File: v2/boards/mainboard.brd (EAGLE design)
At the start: 119.6 x 119.8 mm, 197 parts, among them IC1 LM2596S-ADJ, IC10 DRV8835, IC11 TSOP324, IC12 ESP-WROOM-32, IC13 PAM8403, IC15 MC1525, IC16 INA282, IC17 INA282, IC18 INA282, IC19 INA282, IC2 LM2596S-5.0, IC20 MCP3008, IC3 LD1117A, IC4 LM393, IC7 PCA9634, IC8 PCA9554, IC9 PCA9634, J1 Bat_In, J10 SPI_0, J11 SPI_2, J12 SPI_2, J13 I2C_0, J14 I2C_1, J15 I2C_3, J16 BNO055, J17 Uart_2, J18 Uart_5, J19 Uart_6 (LP), J2 Erw_Pwr, J20 BPS, J21 Servo_2, J22 Servo_3, J23 Erw_Servo, J24 Erw_PWM, J25 ESP32_Uart, J26 SPEAKER_L, J27 SPEAKER_R, J28 AUDIO_TEENSY, J29 SWD, J3 I2C0_5V, J30 SWD_KL02, J31 Erw_ENA, J32 Erw_GPIO, J33 Erw_analog, J34 RC5, J35 ESP32_PROG, J36 SPI1, J4 I2C3_5V, J5 Servo_1, J6 H-Bridge Mode, J7 ESP32_GPIO, J8 SPI_0, J9 SPI_0, SW1 TL32PO, U1 IRLU024N, U5 BS108, U6 BS108, U7 BS108, U8 BS108, U9 BS108, X1 max. 18V

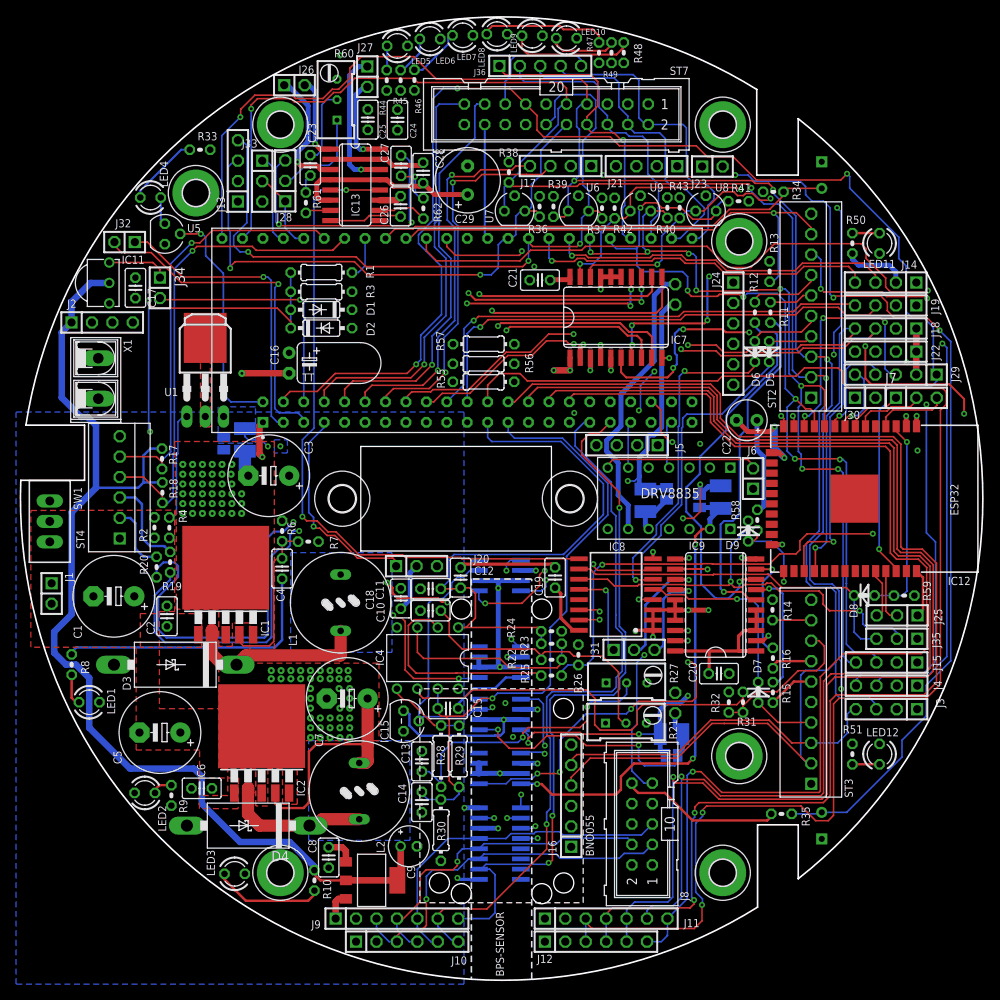
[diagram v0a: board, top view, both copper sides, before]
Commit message: schematics and board files for ct-Bot v2 prototype
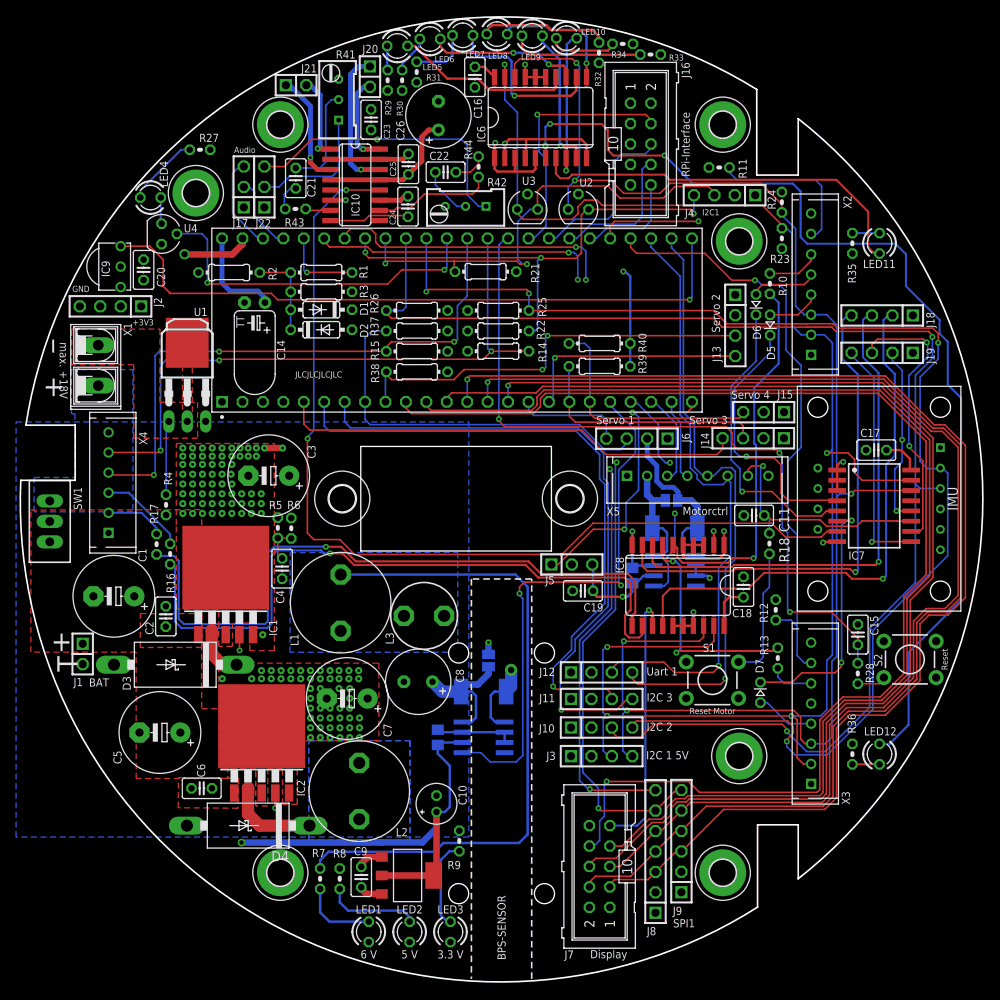
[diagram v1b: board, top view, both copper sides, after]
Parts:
- removed C27: 470nF, rcl:C025-025X050
- removed C28: 1uF, rcl:C025-025X050
- removed C29: 470uF, rcl:E3,5-8
- removed D8, D9: BAT42, ct-bot:0207/2V
- removed IC11: TSOP324, ct-bot:TSOP324
- removed IC12: ESP-WROOM-32, ct-bot:ESP-WROOM-32
- removed IC13: PAM8403, ct-bot:SOP-16
- removed IC15: MC1525, ct-bot:TO92
- removed IC16, IC17, IC18, IC19: INA282, ct-bot:SO08
- removed IC20: MCP3008, ct-bot:SO16
- removed J23: Erw_Servo, ct-bot:1X02
- removed J24: Erw_PWM, ct-bot:1X06
- removed J25: ESP32_Uart, ct-bot:1X03
- removed J26: SPEAKER_L, ct-bot:1X02
- removed J27: SPEAKER_R, ct-bot:1X02
- removed J28: AUDIO_TEENSY, ct-bot:1X03
- removed J29: SWD, ct-bot:1X05
- removed J30: SWD_KL02, ct-bot:1X02
- removed J31: Erw_ENA, ct-bot:1X03
- removed J32: Erw_GPIO, ct-bot:1X02
- removed J33: Erw_analog, ct-bot:1X03
- removed J34: RC5, ct-bot:1X02
- removed J35: ESP32_PROG, ct-bot:1X03
- removed J36: SPI1, ct-bot:1X05
- removed LDR1, LDR2: (no value), ct-bot:SNR2-3.0
- removed R45: 3k9, rcl:0204V
- removed R46: 220, rcl:0204V
- removed R47: 590, rcl:0204V
- removed R48: 115, rcl:0204V
- removed R49: 1k8, rcl:0204V
- removed R50, R51: 4k7, rcl:0204V
- removed R52, R53, R54: 20m, rcl:R1210
- removed R55, R56, R57: 4k7, rcl:0204/7
- removed R58, R59, R61, R62: 10k, rcl:0204V
- removed R60: 5k, ct-bot:RTRIM64W
- removed SJ3, SJ4: (no value), jumper:SJ
- removed ST1: CTBOT_MCU_BRD, ct-bot:DIP66
- removed ST2: Sensoren L, ct-bot:TS_PS25_10
- removed ST3: Sensoren R, ct-bot:TS_PS25_10
- removed ST4: Liniensensoren, ct-bot:TS_PS25_6
- removed ST5: Motor R, ct-bot:1X02/90
- removed ST6: Motor L, ct-bot:1X02/90
- removed ST7: RPI_Interface, con-harting-ml:ML20
- removed U5, U6, U7, U8, U9: BS108, ct-bot:SOT54E
- added IC5: (no value), ct-bot:SO08
- added IC6: PCA9634, ct-bot:SO20W
- added L3: 3u3, ct-bot:FASTRON_07HCP_INDUCTOR
- added MCU: CTBOT_MCU_BRD_V2, ct-bot:DIP48
- added S1, S2: Reset, SparkFun-Switches:TACTILE_SWITCH_PTH_6.0MM
- added U$10: IMU, ct-bot:NXP_9DOF
- added U2, U3, U4: BS108, ct-bot:SOT54E
- added X2: Sensoren L, ct-bot:B8B-XH
- added X3: Sensoren R, ct-bot:B8B-XH
- added X4: Liniensensoren, ct-bot:B6B-XH
- added X5: Motorctrl, ct-bot:B8B-XH
- C10: value 100nF -> 10uF; device rcl:C025-025X050 -> rcl:E2-5
- C11: value 2.2nF -> 1nF
- C12: value 6.8nF -> 100nF; device rcl:C025-025X050 -> rcl:C0805
- C13: device rcl:C025-025X050 -> rcl:C0805
- C14: value 2.2nF -> 10uF; device rcl:C025-025X050 -> rcl:TT2D5L
- C15: value 6.8nF -> 1nF
- C16: value 10uF -> 100nF; device rcl:TT2D5L -> rcl:C025-025X050
- C21: value 100nF -> 470nF
- C22: value 10uF -> 470nF; device rcl:E2,5-5 -> rcl:C025-025X050
- C23: value 470nF -> 1uF
- C24: value 1uF -> 100nF
- C26: value 100nF -> 470uF; device rcl:C025-025X050 -> rcl:E3,5-8
- C3: value 220u -> 220uF
- C7: value 680uF -> 220uF
- C8: value 100nF -> 180uF; device rcl:C025-025X050 -> rcl:E3,5-8
- C9: value 10uF -> 100nF; device rcl:E2-5 -> rcl:C025-025X050
- IC10: value DRV8835 -> PAM8403; device ct-bot:DRV8835 -> ct-bot:SOP-16
- IC4: value LM393 -> (none); device linear:DIL08 -> ct-bot:SO08
- IC7: value PCA9634 -> PCA9554; device ct-bot:SO20W -> ct-bot:SO16W
- IC8: value PCA9554 -> PCA9634; device ct-bot:SO16W -> ct-bot:SO20W
- IC9: value PCA9634 -> TSOP324; device ct-bot:SO20W -> ct-bot:TSOP324
- J10: value SPI_0 -> I2C_2; device ct-bot:1X06 -> ct-bot:1X04
- J11: value SPI_2 -> I2C_3; device ct-bot:1X07 -> ct-bot:1X04
- J12: value SPI_2 -> Uart_1; device ct-bot:1X06 -> ct-bot:1X04
- J13: value I2C_0 -> Servo_2
- J14: value I2C_1 -> Servo_3
- J15: value I2C_3 -> Servo_4; device ct-bot:1X04 -> ct-bot:1X03
- J16: value BNO055 -> RPi_Interface; device ct-bot:1X06 -> con-harting-ml:ML10
- J17: value Uart_2 -> Audio; device ct-bot:1X04 -> ct-bot:1X03
- J18: value Uart_5 -> Erw_DRV
- J19: value Uart_6 (LP) -> Erw_ENA
- J20: value BPS -> SPEAKER_R; device ct-bot:1X03 -> ct-bot:1X02
- J21: value Servo_2 -> SPEAKER_L; device ct-bot:1X04 -> ct-bot:1X02
- J22: value Servo_3 -> AUDIO_IN; device ct-bot:1X04 -> ct-bot:1X03
- J3: value I2C0_5V -> I2C1_5V
- J4: value I2C3_5V -> I2C_1
- J5: value Servo_1 -> BPS; device ct-bot:1X04 -> ct-bot:1X03
- J6: value H-Bridge Mode -> Servo_1; device ct-bot:1X02 -> ct-bot:1X04
- J7: value ESP32_GPIO -> SPI_1; device ct-bot:1X03 -> con-harting-ml:ML10
- J8: value SPI_0 -> SPI_1; device con-harting-ml:ML10 -> ct-bot:1X07
- J9: value SPI_0 -> SPI_1; device ct-bot:1X07 -> ct-bot:1X06
- R10: value 120 -> 180
- R11, R12: value 180 -> 47k
- R13, R17: value 47k -> 180
- R14, R2, R37: device rcl:0204V -> rcl:0204/7
- R15: value 180 -> 47k; device rcl:0204V -> rcl:0204/7
- R18: value 47k -> 330
- R19: value 180 -> 30m; device rcl:0204V -> rcl:R2512
- R20: value 180 -> 100m; device rcl:0204V -> rcl:R2512
- R21: value 5k -> 4k7; device ct-bot:RTRIM64W -> rcl:0204/7
- R22, R38, R39: value 10k -> 4k7; device rcl:0204V -> rcl:0204/7
- R23: value 1M -> 10k
- R25: value 10k -> 1k1; device rcl:0204V -> rcl:0204/7
- R26: value 15k -> 1k1; device rcl:0204V -> rcl:0204/7
- R27: value 5k -> 1k8; device ct-bot:RTRIM64W -> rcl:0204V
- R28: value 10k -> 330; device rcl:0204/7 -> rcl:0204V
- R29: value 1M -> 27k; device rcl:0204/7 -> rcl:0204V
- R30: device rcl:0204/7 -> rcl:0204V
- R31: value 10k -> 15k
- R32: value 15k -> 2k2
- R33: value 100 -> 2k2
- R34: value 470k -> 1k8
- R35: value 470k -> 10k
- R36, R44: value 4k7 -> 10k
- R40: value 1k1 -> 4k7; device rcl:0204V -> rcl:0204/7
- R41: value 1k1 -> 5k; device rcl:0204V -> ct-bot:RTRIM64W
- R42: value 1k8 -> 5k; device rcl:0204V -> ct-bot:RTRIM64W
- R43: value 1k8 -> 10k
- R5: value 20m -> 3k9 0.1%; device rcl:R1210 -> rcl:0204V
- R6: value 3k9 0.1% -> 1k 0.1%
- R7: value 1k 0.1% -> 27k
- R8: value 390 -> 22k
- R9: value 330 -> 15k
- moved C17 94.3 mm to (46.6, 6.05), turned to 180 degrees
- moved R30 93.3 mm to (-12.4, 52.0), turned to 90 degrees
- moved R10 93.3 mm to (33.4, 26.7), turned to 270 degrees
- moved R31 88.2 mm to (-10.6, 53.0), turned to 90 degrees
- moved C20 87.4 mm to (-44.5, 28.4), turned to 270 degrees
- moved IC9 85.1 mm to (-47.3, 28.9), turned to 270 degrees
- moved R27 84.6 mm to (-37.5, 43.4), turned to 0 degrees
- moved R29 84.5 mm to (-14.2, 52.0), turned to 90 degrees
- moved R32 82.3 mm to (12.1, 55.4)
- moved J16 81.5 mm to (17.3, 44.1), turned to 270 degrees
- moved J22 79.9 mm to (-29.5, 38.8), turned to 90 degrees
- moved R36 78.4 mm to (43.6, -31.8), turned to 270 degrees
- moved R16 76.0 mm to (-41.2, -6.87)
- moved R18 75.7 mm to (33.3, -5.58)
- moved R35 71.5 mm to (43.6, 31.8), turned to 90 degrees
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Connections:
- net V5_L1 renamed V5_L2
- removed net A22_DAC1: J33.1, ST1.48
- removed net AUDIO_OUT: J28.1, J33.2, ST1.49
- removed net BAT_CUR: IC17.5, IC20.1
- removed net BNO055_RESET: IC8.7, J16.6
- removed net DRV_RADLED_L: IC9.6, R11.2
- removed net DRV_RADLED_R: IC9.7, R15.1
- removed net EN: D8.1, IC12.3, R59.1
- removed net ENC_L: R25.2, R26.1, ST2.8
- removed net ENC_R: R31.2, R32.1, ST3.8
- removed net ESP32_PROG: D9.2, IC8.11, J35.2
- removed net ESP32_RESET: D8.2, IC8.10, J35.3
- removed net GND_BAT: IC17.1, R5.2, SJ1.2, U1.3
- removed net GPIO_24: J32.1, ST1.2
- removed net GPIO_46: J32.2, ST1.3
- removed net IO0: D9.1, IC12.25, R58.2
- removed net IO10: IC12.18
- removed net IO11: IC12.19
- removed net IO13: IC12.16
- removed net IO15: IC12.23
- removed net IO18: IC12.30
- removed net IO19: IC12.31
- removed net IO21: IC12.33
- removed net IO34: IC12.6, J7.2
- removed net IO35: IC12.7, J7.1
- removed net IO36: IC12.4, J7.3
- removed net IO39: IC12.5
- removed net IO4: IC12.26
- removed net IO5: IC12.29
- removed net IO6: IC12.20
- removed net IO7: IC12.21
- removed net IO8: IC12.22
- removed net IO9: IC12.17
- removed net KL02_DC: IC12.14, J30.1
- removed net KL02_DD: IC12.13, J30.2
- removed net LDR_L: LDR1.2, R34.1, ST1.53
- removed net LDR_R: LDR2.2, R35.1, ST1.56
- removed net MCP_CH4: IC20.5
- removed net MCP_CH5: IC20.6
- removed net MCP_CH6: IC20.7
- removed net MCP_CH7: IC20.8
- removed net MOT_L_1: IC10.AOUT1, ST6.1
- removed net MOT_L_2: IC10.AOUT2, IC18.8, R53.1, SJ3.1
- removed net MOT_L_CUR: IC18.5, IC20.2
- removed net MOT_L_DIR: IC10.APHASE, ST1.19
- removed net MOT_L_PWM: IC10.AENBL, ST1.20
- removed net MOT_L_SENS: IC18.1, R53.2, SJ3.2, ST6.2
- removed net MOT_R_1: IC10.BOUT1, ST5.1
- removed net MOT_R_2: IC10.BOUT2, IC19.8, R52.1, SJ2.1
- removed net MOT_R_CUR: IC19.5, IC20.3
- removed net MOT_R_DIR: IC10.BPHASE, ST1.21
- removed net MOT_R_PWM: IC10.BENBL, ST1.22
- removed net MOT_R_SENS: IC19.1, R52.2, SJ2.2, ST5.2
- removed net N$10: IC4.6, R31.1
- removed net N$3: IC10.MODE, J6.2
- removed net N$34: C10.1, R21.2, R22.1
- removed net N$35: IC4.3, R22.2, R23.1
- removed net N$36: C13.1, R27.2, R28.1
- removed net N$37: IC4.5, R28.2, R29.1
- removed net N$45: R15.2, ST3.6
- removed net N$47: R11.1, ST2.6
- removed net PWM_ERW_1: J24.1, ST1.39
- removed net PWM_ERW_2: J24.2, ST1.40
- removed net PWM_ERW_3: J24.3, J8.9, ST1.42
- removed net PWM_ERW_4: J24.4, ST1.41
- removed net PWM_ERW_5: J24.5, ST1.43
- removed net PWM_ERW_6: J24.6, ST1.44
- removed net RAD_L: C11.1, C12.1, IC4.1, R23.2, R24.1, ST1.12
- removed net RAD_R: C14.1, C15.1, IC4.7, R29.2, R30.1, ST1.13
- removed net RC5: IC11.1, J34.1
- removed net REF_2.5: IC15.2, IC18.3, IC19.3, IC20.15
- removed net RPI_3V3: ST7.11
- removed net RPI_SPI0_CE1: J36.5, ST7.15
- removed net RX5: IC12.28, J18.4, ST1.30
- removed net RX6: J19.4, ST1.32
- removed net RXD0: IC12.34, J25.3
- removed net SCL0: J13.4, R37.1, ST1.60, ST7.12, U6.S
- removed net SCL0_5V: IC8.14, J16.5, J3.4, R39.1, ST1.45, ST2.3, ST3.3, ST7.7, U6.D
- removed net SCL3_5V: IC7.18, IC9.18, J4.4, R43.1, U8.D
- removed net SDA0: J13.3, R36.1, ST1.59, ST7.10, U7.S
- removed net SDA0_5V: IC8.15, J16.4, J3.3, R38.1, ST1.46, ST2.2, ST3.2, ST7.9, U7.D
- removed net SDA3_5V: IC7.19, IC9.19, J4.3, R42.1, U9.D
- removed net SERVO5_PWM: IC20.10, J23.2, J9.7, ST1.18
- removed net SERVO_CUR: IC16.5, IC20.4
- removed net SERVO_PWR: IC16.1, J21.2, J22.2, J5.2, R54.2, SJ4.2, ST7.1
- removed net SPI0_CS0: J8.6, ST1.8
- removed net SPI0_CS4: J8.7, ST1.9
- removed net SPI0_CS5: J8.8, ST1.10
- removed net SPI0_MISO: IC20.12, J10.4, J8.4, J9.4, ST1.6
- removed net SPI0_MOSI: IC20.11, J10.3, J8.3, J9.3, ST1.5
- removed net SPI0_SCK: IC20.13, J10.5, J8.5, J9.5, ST1.7
- removed net SPI1_CS0: J36.4, ST1.68, ST7.2
- removed net SPI2_CS0: J11.6, ST1.37
- removed net SWCLK: IC12.9, J29.4
- removed net SWDIO: IC12.8, J29.5
- removed net SWD_EN: IC12.12, J29.3
- removed net TX5: IC12.27, J18.3, ST1.31
- removed net TX6: J19.3, ST1.33
- removed net TXD0: IC12.35, J25.2
- removed net VCC: C16.+, C19.1, C20.1, C21.1, C24.1, C25.1, C28.1, C29.+, C7.+, C8.1, IC10.VCC, IC13.13, IC13.4, IC13.6, IC2.4, IC3.VIN, IC7.1, IC7.20, IC7.3, IC7.5, IC8.16, IC9.1, IC9.20, IC9.3, IC9.4, IC9.5, J10.1, J11.2, J12.2, J13.2, J14.2, J15.2, J16.1, J17.2, J18.2, J19.2, J2.2, J3.2, J4.2, J6.1, J8.1, J9.1, L2.2, R38.2, R39.2, R42.2, R43.2, R44.1, R45.1, R46.1, R47.1, R48.1, R49.1, R50.1, R51.1, R9.2, ST1.1, ST2.1, ST3.1, ST4.1, ST7.5
- new net +5V: C14.+, C16.1, C17.1, C18.1, C23.1, C25.1, C26.+, C9.1, IC10.13, IC10.4, IC10.6, IC3.VIN, IC4.1, IC6.1, IC6.20, IC6.3, IC6.5, IC7.16, IC8.1, IC8.20, IC8.3, IC8.4, IC8.5, J10.2, J11.2, J12.2, J16.7, J2.2, J3.2, J4.2, J7.1, J8.1, J9.1, MCU.48, R19.2, R23.2, R24.2, R27.2, R29.1, R30.1, R31.1, R32.1, R33.1, R34.1, R35.1, R36.1, R8.2, SJ1.2, X2.P$1, X3.P$1, X4.P$1, X5.P$1
- new net 5V_SUPPLY: C8.+, IC4.8, L3.2, R19.1, SJ1.1
- new net 6V_SERVO: IC5.1, J13.2, J14.2, J15.2, J16.9, J6.2, R20.2, SJ2.2
- new net AUDIO_L: J17.2, MCU.45
- new net AUDIO_R: J17.3, MCU.46
- new net CURRENT_5V: IC4.5, MCU.20
- new net CURRENT_SERVO: IC5.5, MCU.21
- new net DRV_DISPLAY: IC8.13, J7.9
- new net DRV_ERW_3: IC8.14, J18.2
- new net ENA_ERW_2: IC7.10, J19.3
- new net GPIO1: J8.6, J9.6, MCU.42
- new net GPIO2: J8.7, MCU.43
- new net IMU_RST: IC7.12, J19.2, U$10.RST
- new net MCTRL_RESET: C11.1, IC7.11, R18.2, X5.P$7
- new net N$14: R28.1, S2.3
- new net N$39: C22.2, R42.2
- new net SCL1_5V: IC6.18, IC7.14, IC8.18, J3.4, R24.1, U2.D, X2.P$3, X3.P$3
- new net SCL2: J10.3, MCU.39, R26.1, U$10.SCL
- new net SDA1_5V: IC6.19, IC7.15, IC8.19, J3.3, R23.1, U3.D, X2.P$2, X3.P$2
- new net SDA2: J10.4, MCU.38, R25.1, U$10.SDA
- new net SERVO3_FB: J14.4, MCU.5
- new net SPI1_CS1: J7.6, MCU.12
- new net SPI1_CS2: J7.7, MCU.11
- new net SPI1_CS3: J7.8, MCU.10
- new net V5_L3: C7.+, IC2.4, L2.2, L3.1
- new net VCC_MCU: MCU.3
- net +3V3: now also C10.+, C12.1, C13.1, C19.1, C20.1, IC4.6, IC5.6, IC9.2, J16.5, J5.3, J7.10, MCU.47, R11.2, R12.1, R14.2, R15.2, R21.2, R22.2, R25.2, R38.2, R39.2, R9.2, U$10.VIN, U2.G, U3.G; no longer C17.1, C18.1, C22.+, C9.+, IC11.2, IC12.2, IC15.3, IC16.6, IC17.6, IC18.6, IC19.6, IC20.16, IC4.8, J20.3, J8.10, R10.2, R13.2, R14.1, R17.2, R18.2, R21.3, R24.2, R27.3, R30.2, R32.2, R33.2, R34.2, R35.2, R36.2, R41.2, R55.2, R56.2, R57.2, R58.1, R59.2, ST7.3, U6.G, U7.G, U8.G, U9.G
- net +6V: now also IC5.8, R20.1, R5.2, R7.1, SJ2.1, X5.P$2; no longer IC10.VIN, IC16.8, J2.3, R54.1, R6.2, R8.1, SJ4.1
- net ABST_SHDN_L: now also IC7.4; no longer IC8.4
- net ABST_SHDN_R: now also IC7.6; no longer IC8.5
- net AGND: now also C23.2, C24.2, IC10.11, J17.1, J22.1, MCU.2, R41.3, R42.3; no longer C25.2, C26.2, IC13.11, IC15.1, IC16.2, IC16.3, IC16.7, IC17.2, IC17.3, IC17.7, IC18.2, IC18.7, IC19.2, IC19.7, IC20.14, J33.3, R60.3, ST1.47
- net BAT_IN: now also J16.3
- net BAT_IN_FB: now also MCU.44; no longer ST1.52
- net BPS: now also J5.1, MCU.24; no longer J20.1, ST1.4
- net DEBUG_LED: now also MCU.37, U4.G; no longer ST1.23, U5.G
- net DRV_ERW_1: now also IC8.9, J18.4; no longer IC9.13, J31.2
- net DRV_ERW_2: now also IC8.8, J18.3; no longer IC9.14, J31.3
- net DRV_KANTLED_L: now also IC8.6, R10.2; no longer IC9.8, R12.2
- net DRV_KANTLED_R: now also IC8.7, R13.1; no longer IC9.9, R16.1
- net DRV_LINE_L: now also IC8.11, R17.2; no longer IC9.11, R20.2
- net DRV_LINE_R: now also IC8.12, R16.2; no longer IC9.12, R19.2
- net ENA_AUDIO: now also IC10.12, IC7.7; no longer IC13.12, IC8.9
- net ENA_ERW_1: now also IC7.9, J19.4; no longer IC8.12, J31.1
- net FERNBED: now also IC9.1, MCU.25; no longer J34.2, ST1.25
- net GND: now also C10.-, C14.-, C16.2, C25.2, C26.-, C8.-, C9.2, IC10.15, IC10.2, IC4.2, IC4.3, IC4.7, IC5.2, IC5.3, IC5.7, IC6.10, IC6.15, IC6.16, IC6.17, IC6.2, IC6.4, IC7.1, IC7.3, IC7.8, IC8.10, IC8.15, IC8.16, IC8.17, IC9.3, J10.1, J16.1, J16.2, J2.3, J5.2, J6.1, J7.2, MCU.1, R6.1, S1.1, S2.1, U$10.GND, U1.3, U4.S, X2.P$8, X3.P$8, X4.P$6, X5.P$8; no longer C10.2, C14.2, C16.-, C21.2, C22.-, C24.2, C28.2, C29.-, C8.2, C9.-, IC10.LGND, IC10.MGND, IC11.3, IC12.1, IC12.15, IC12.24, IC12.38, IC13.15, IC13.2, IC17.8, IC20.9, IC4.4, IC7.10, IC7.15, IC7.16, IC7.17, IC7.4, IC8.1, IC8.3, IC8.8, IC9.10, IC9.15, IC9.16, IC9.17, IC9.2, J10.2, J16.3, J17.1, J20.2, J21.1, J22.1, J25.1, J29.2, J35.1, J5.1, LDR1.1, LDR2.1, R21.1, R27.1, R5.1, R7.1, SJ1.1, ST1.11, ST2.10, ST3.10, ST4.6, ST7.20, U5.S
- net KANTE_L: now also MCU.29, R11.1, X2.P$7; no longer R13.1, ST1.54, ST2.9
- net KANTE_R: now also MCU.28, R12.2, X3.P$7; no longer R14.2, ST1.55, ST3.9
- net LINE_IN_L: now also J22.2, R41.1; no longer J28.2, R60.1
- net LINE_IN_R: now also J22.3, R42.1; no longer C27.2, J28.3
- net LINIE_L: now also MCU.36, R15.1, X4.P$4; no longer R18.1, ST1.51, ST4.4
- net LINIE_R: now also MCU.35, R14.1, X4.P$5; no longer R17.1, ST1.50, ST4.5
- net N$1: now also R16.1, X4.P$3; no longer R19.1, ST4.3
- net N$11: now also R8.1; no longer R9.1
- net N$13: now also IC6.8; no longer IC7.8
- net N$15: now also IC6.9; no longer IC7.9
- net N$16: now also IC6.11; no longer IC7.11
- net N$17: now also IC6.12; no longer IC7.12
- net N$18: now also IC6.13; no longer IC7.13
- net N$19: now also IC6.14; no longer IC7.14
- net N$2: now also R9.1; no longer R10.1
- net N$20: now also R29.2; no longer R44.2
- net N$21: now also R30.2; no longer R45.2
- net N$22: now also R31.2; no longer R46.2
- net N$23: now also R32.2; no longer R47.2
- net N$24: now also R33.2; no longer R48.2
- net N$25: now also R34.2; no longer R49.2
- net N$26: now also R35.2; no longer R50.2
- net N$27: now also R36.2; no longer R51.2
- net N$28: now also R27.1; no longer R33.1
- net N$29: now also U4.D; no longer U5.D
- net N$30: now also R17.1, X4.P$2; no longer R20.1, ST4.2
- net N$31: now also IC10.1, J21.2; no longer IC13.1, J26.2
- net N$32: now also IC10.3, J21.1; no longer IC13.3, J26.1
- net N$33: now also C24.1, IC10.8; no longer C26.1, IC13.8
- net N$40: now also IC10.7, R43.1; no longer IC13.7, R61.1
- net N$41: now also C21.1, R43.2; no longer C23.1, R61.2
- net N$42: now also C21.2, R41.2; no longer C23.2, R60.2
- net N$43: now also IC10.14, J20.1; no longer IC13.14, J27.1
- net N$44: now also IC10.16, J20.2; no longer IC13.16, J27.2
- net N$46: now also IC10.10, R44.1; no longer IC13.10, R62.1
- net N$48: now also C22.1, R44.2; no longer C27.1, R62.2
- net N$5: now also R18.1, S1.3; no longer IC4.2, R25.1
- net N$51: now also R10.1, X2.P$6; no longer R12.1, ST2.7
- net N$53: now also R13.2, X3.P$6; no longer R16.2, ST3.7
- net N$6: now also IC6.6; no longer IC7.6
- net N$7: now also IC6.7; no longer IC7.7
- net N$8: now also R7.2; no longer R8.2
- net N$9: now also R5.1, R6.2; no longer R6.1, R7.2
- net RESET: now also C15.1, MCU.34, R28.2; no longer IC12.36, J29.1, ST1.24, ST7.13
- net RX1: now also J12.4, MCU.26, X5.P$5; no longer ST1.26, ST7.19
- net RX2: now also MCU.22, X5.P$3; no longer J17.4, ST1.28
- net SCHRANKE_SHDN: now also IC7.5; no longer IC8.6
- net SCL1: now also J4.4, MCU.41, R22.1, U2.S; no longer J14.4, ST1.61
- net SCL3: now also J11.3, MCU.6; no longer IC12.11, J15.3, R41.1, ST1.64, U8.S
- net SDA1: now also J4.3, MCU.40, R21.1, U3.S; no longer J14.3, ST1.62
- net SDA3: now also J11.4, MCU.7; no longer IC12.10, J15.4, R40.1, ST1.63, U9.S
- net SERVO1_FB: now also J6.4, MCU.16; no longer J5.4, ST1.57
- net SERVO1_PWM: now also J6.3, MCU.8, R37.1; no longer J5.3, R55.1, ST1.14
- net SERVO2_FB: now also J13.4, MCU.17; no longer J21.4, ST1.58, ST7.18
- net SERVO2_PWM: now also J13.3, MCU.9, R38.1; no longer J21.3, R56.1, ST1.15, ST7.16
- net SERVO3_PWM: now also J14.3, MCU.18, R39.1; no longer J22.3, R57.1, ST1.16, ST7.14
- net SERVO4_PWM: now also J15.3, MCU.19, R40.1; no longer J10.6, J23.1, J9.6, ST1.17
- net SPI1_MISO: now also J7.4, J8.4, J9.4, MCU.14; no longer J36.2, ST1.66, ST7.6
- net SPI1_MOSI: now also J7.3, J8.3, J9.3, MCU.13; no longer J36.1, ST1.65, ST7.8
- net SPI1_SCK: now also J7.5, J8.5, J9.5, MCU.15; no longer J36.3, ST1.67, ST7.4
- net SPI2_CS1: now also J16.4, MCU.33; no longer J11.7, J12.6, ST1.38
- net SPI2_MISO: now also J16.8, MCU.31; no longer J11.4, J12.4, ST1.35
- net SPI2_MOSI: now also J16.6, MCU.32; no longer J11.3, J12.3, ST1.34
- net SPI2_SCK: now also J16.10, MCU.30; no longer J11.5, J12.5, ST1.36
- net TX1: now also J12.3, MCU.27, X5.P$6; no longer ST1.27, ST7.17
- net TX2: now also MCU.23, X5.P$4; no longer J17.3, ST1.29
- net VL53L0X_SHUT_L: now also X2.P$4; no longer ST2.4
- net VL53L0X_SHUT_R: now also X3.P$4; no longer ST3.4
- net VL6180X_SHDN: now also X2.P$5; no longer ST2.5
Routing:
- net SDA0_5V: track 266.4 -> 0.00 mm, vias 4 -> 0
- net SCL0_5V: track 251.4 -> 0.00 mm, vias 6 -> 0
- net +3V3: track 616.2 -> 400.2 mm, vias 7 -> 4
- net SPI0_MOSI: track 213.2 -> 0.00 mm, vias 1 -> 0
- net SPI0_MISO: track 208.2 -> 0.00 mm, vias 1 -> 0
- net SDA1_5V: track 0.00 -> 201.5 mm, vias 0 -> 5
- net SPI0_SCK: track 197.0 -> 0.00 mm
- net SERVO_PWR: track 194.6 -> 0.00 mm, vias 9 -> 0
- net SCL1_5V: track 0.00 -> 193.7 mm, vias 0 -> 5
- net SCL2: track 0.00 -> 170.7 mm, vias 0 -> 2
- net SDA2: track 0.00 -> 165.2 mm, vias 0 -> 4
- net LDR_R: track 159.7 -> 0.00 mm, vias 5 -> 0
- net SPI1_CS3: track 0.00 -> 157.8 mm, vias 0 -> 1
- net SPI2_MOSI: track 178.0 -> 21.6 mm, vias 2 -> 0
- net SPI0_CS0: track 153.1 -> 0.00 mm
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- added copper zone on layer 15, net +5V
- added copper zone on layer 16, net BAT+
- removed copper zone on layer 15, net +6V
- removed copper zone on layer 16, net AGND
- removed copper zone on layer 15, net BAT+
- removed copper zone on layer 2, net BAT-
- removed copper zone on layer 16, net GND_BAT
- removed copper zone on layer 15, net VCC
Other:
- board size 119.6 x 119.8 mm -> 119.7 x 120 mm
- board text added: "+"
- board text added: "+3V3"
- board text added: "3.3 V"
- board text added: "5 V"
- board text added: "6 V"
- board text added: "Audio"
- board text added: "BAT"
- board text added: "Display"
- board text added: "GND"
- board text added: "I2C 1 5V"
- board text added: "I2C 2"
- board text added: "I2C 3"
- board text added: "I2C1"
- board text added: "JLCJLCJLCJLC"
- board text added: "Motorctrl"
- board text added: "RPi-Interface"
- board text added: "Reset"
- board text added: "Reset Motor"
- board text added: "SPI1"
- board text added: "Servo 1"
- board text added: "Servo 2"
- board text added: "Servo 3"
- board text added: "Servo 4"
- board text added: "T"
- board text added: "Uart 1"
- board text added: "_"
- board text added: "ct-Bot v2 Mainboard T. Sandmann, CC BY-SA 4.0 v0.9.2 - 08/2022"
- board text added: "max. +18V"
- board text removed: "BNO055"
- board text removed: "ESP32"
